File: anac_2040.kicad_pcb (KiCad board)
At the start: 2 copper layers, 53.2 x 68.2 mm, 62 parts, among them J1 Conn_01x02, J10 Debug, J5 Conn_01x09, J6 Barrel_Jack_MountingPin, J7 USB_C_Receptacle_USB2.0, Q1 PJA3432AU, Q2 PJA3432AU, SW1 SW_Push, SW2 SW_Push, U1 RP2040, U2 W25Q16JVSSIQ, U3 LM4040DBZ-3, U4 AP63203WU, Y1 Crystal_Small

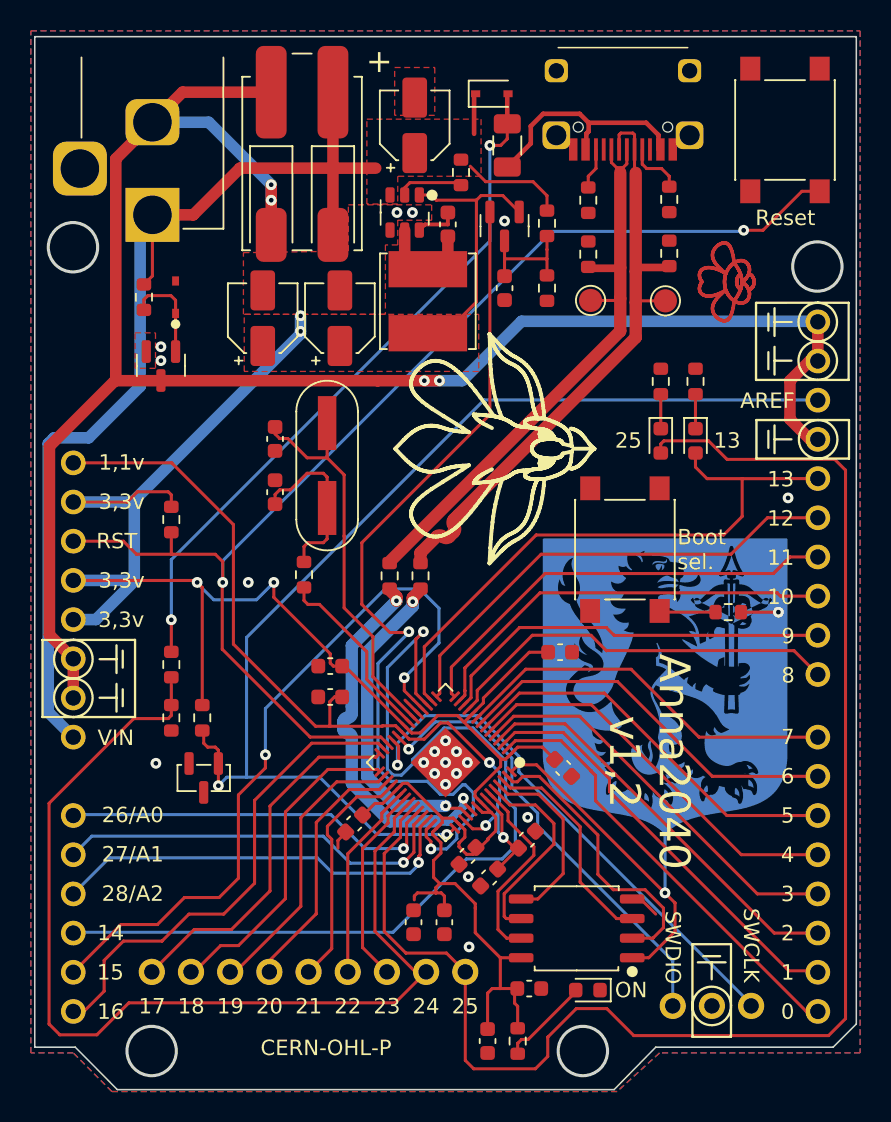
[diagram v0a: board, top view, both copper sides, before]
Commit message: fixed things
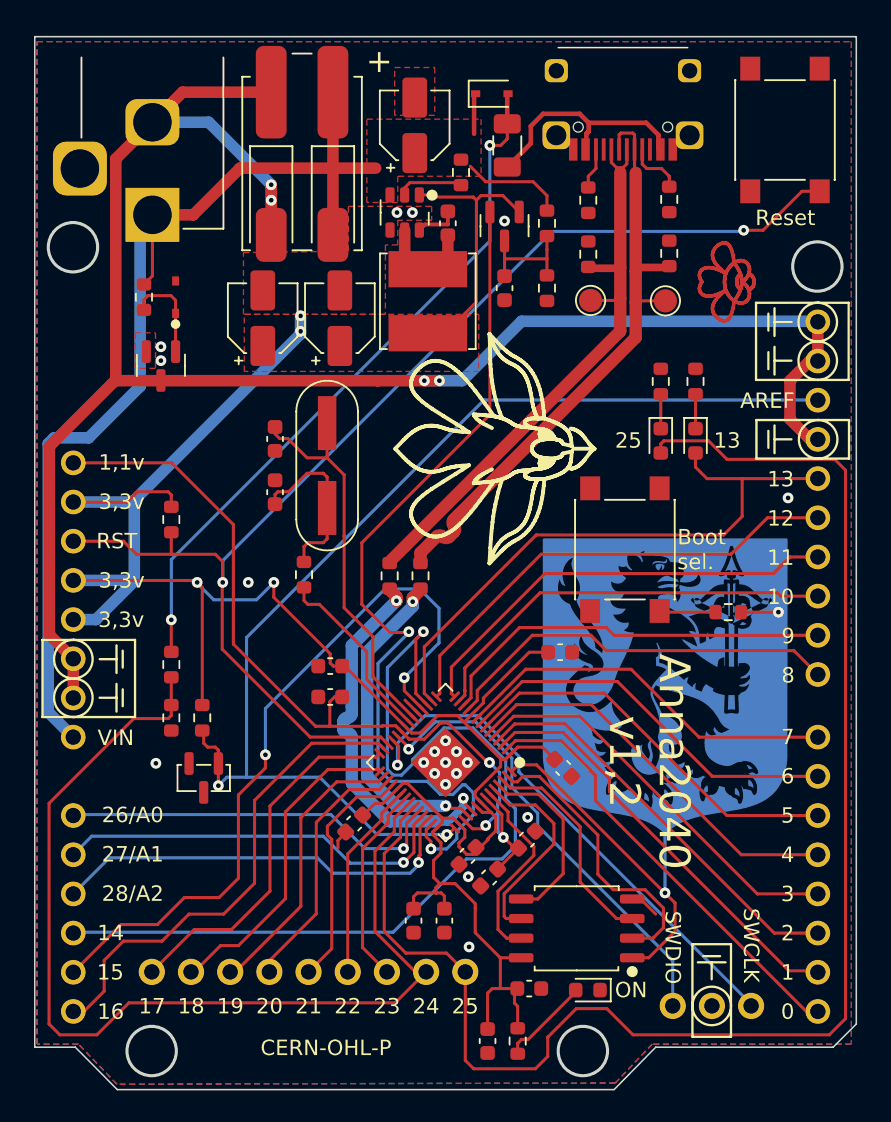
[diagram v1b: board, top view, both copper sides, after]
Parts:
- moved C13 0.10 mm to (152.9, 112.0)
- moved C14 0.10 mm to (154.9, 112.0)
- moved C16 0.07 mm to (155.2, 66.8)
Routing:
- net +3.3V: track 160.2 -> 160.9 mm
